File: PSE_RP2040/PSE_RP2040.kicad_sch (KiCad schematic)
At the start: 68 parts, among them IC2 SAM-M8Q-0, J1 USB_B, J2 USB_B_Micro, J3 8P8C_LED, J4 Conn_01x03, Q1 DTC114Y, Q2 Q_PMOS_GSD, SW1 SW_Push, U1 RP2040, U2 PCF8563T, U3 W25Q32JVSS, U5 W25Q16JVUXIQ, U6 PAM7Q, Y1 Crystal_GND3, Y2 Crystal_GND24

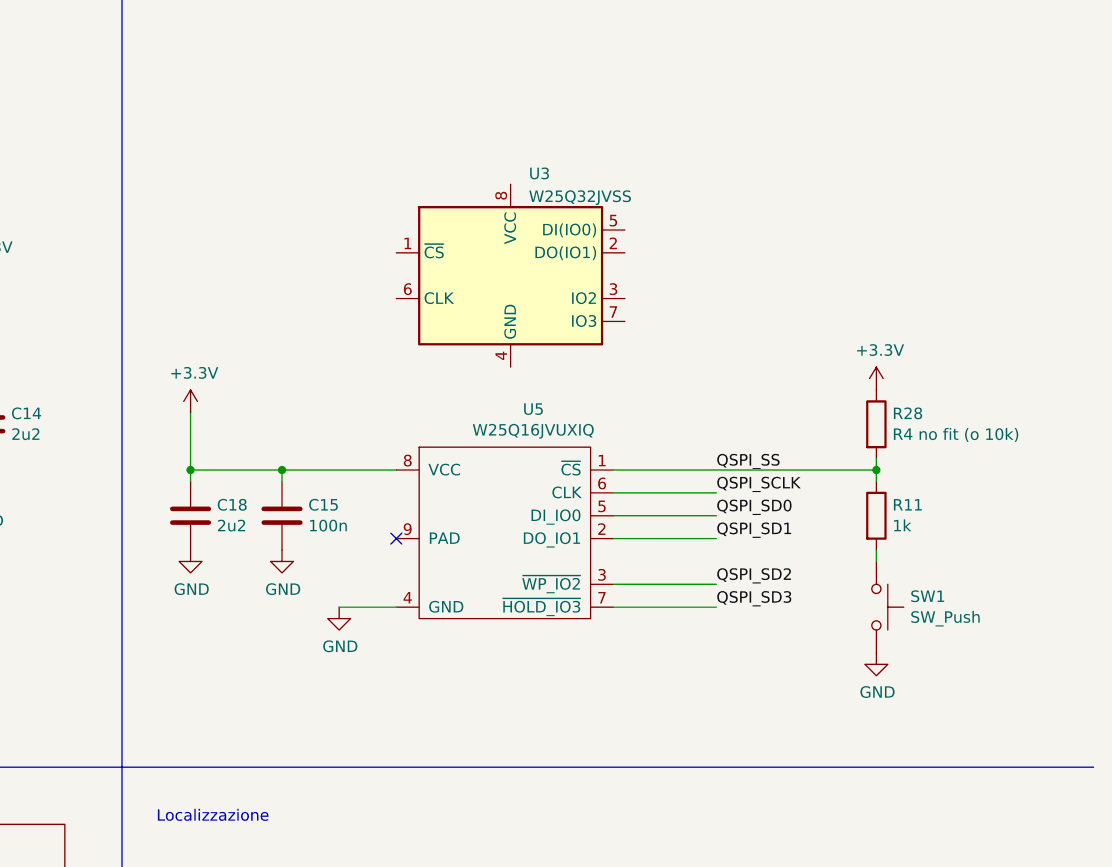
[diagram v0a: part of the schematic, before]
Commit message: footprint flash
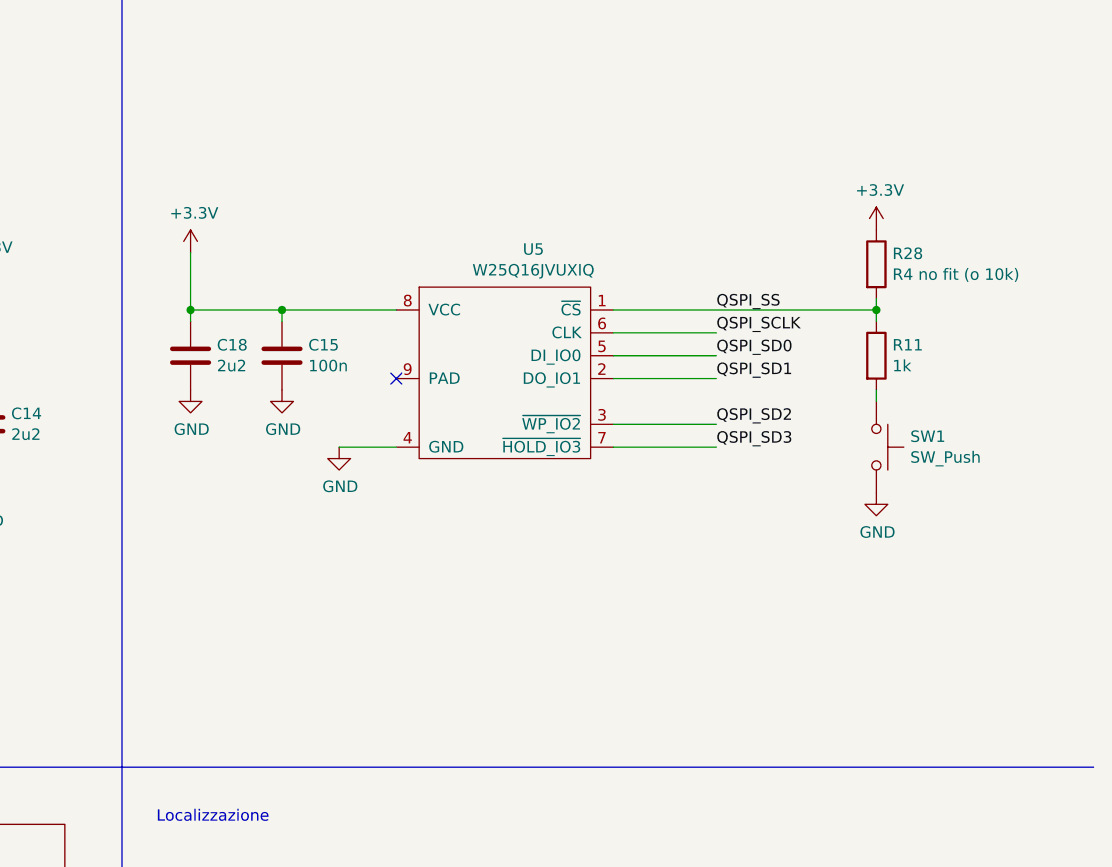
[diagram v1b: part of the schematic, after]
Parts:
- removed U3: W25Q32JVSS, Package_SO:SOIC-8_5.23x5.23mm_P1.27mm, symbol Memory_Flash:W25Q32JVSS
- U6: footprint (none) -> PSE2021:PAM-7Q
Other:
- moved on the sheet: C15, C18, R11, R28, SW1, U5
